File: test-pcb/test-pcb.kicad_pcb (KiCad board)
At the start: 4 copper layers, 16 parts, among them IC1 VNH5019ATR-E, J1 Conn_01x06, J2 Conn_01x06, J3 Conn_01x03, Q1 IPD050N10N5ATMA1

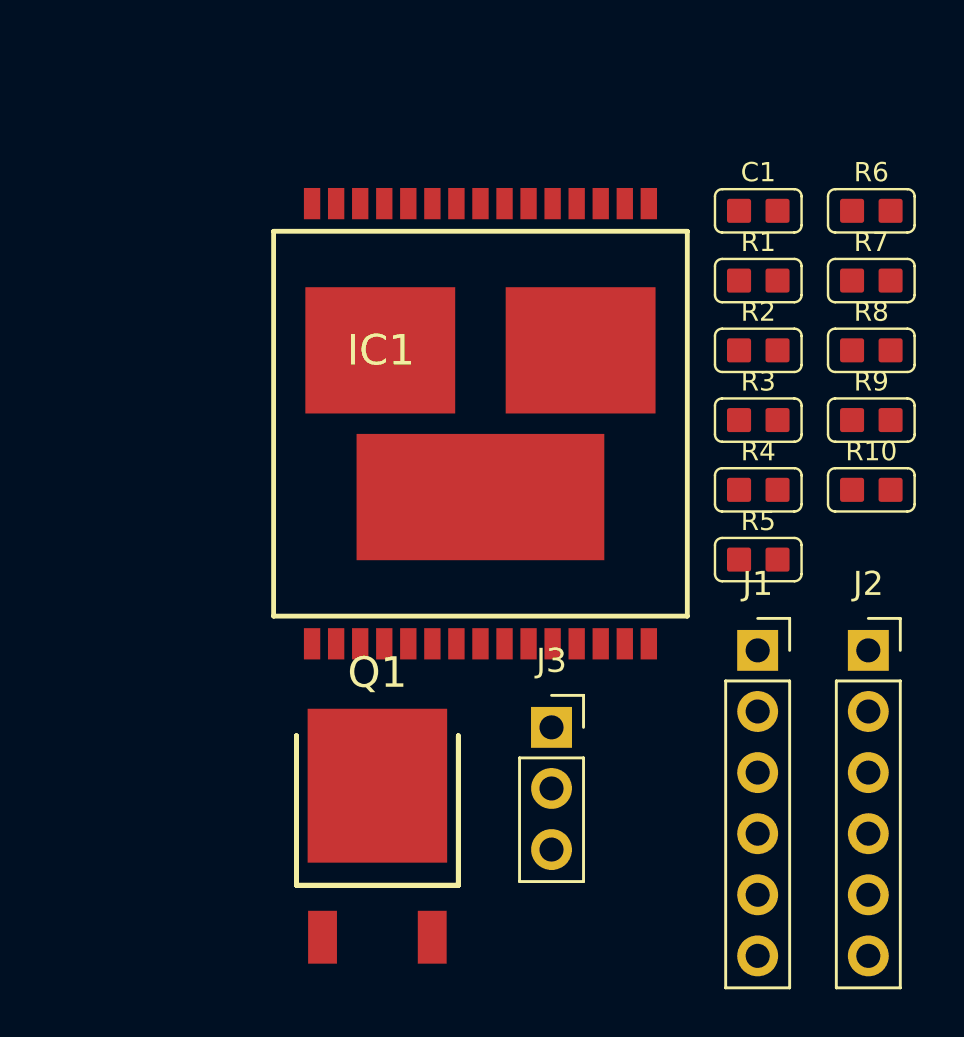
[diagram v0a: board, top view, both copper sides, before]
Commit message: test - thermal vias for driver
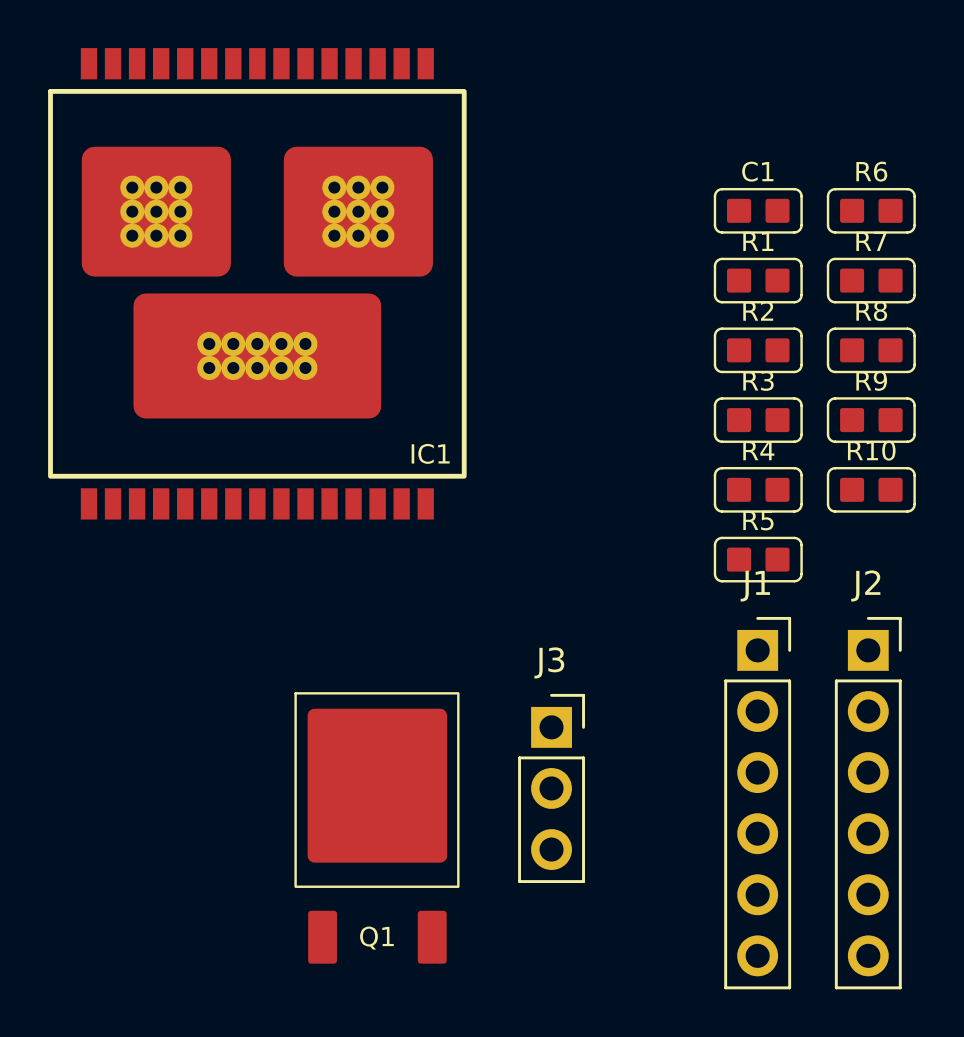
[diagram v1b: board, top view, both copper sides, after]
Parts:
- moved IC1 15.3 mm to (30.5, 35.6)

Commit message: test - fixed mdriver sch
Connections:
- IC1 pad GND: (no net) -> GND
- J2 pad 1: VCC -> /M1 OUTA
- J2 pad 6: GND -> /M1 OUTB
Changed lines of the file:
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@@
     (pad "24" smd rect (at -1 -9.15) (size 0.68 1.3) (layers "F.Cu" "F.Paste" "F.Mask"))
     (pad "29" smd rect (at -6 -9.15) (size 0.68 1.3) (layers "F.Cu" "F.Paste" "F.Mask"))
-    (pad "GND" smd rect (at -5 -9.15) (size 0.68 1.3) (layers "F.Cu" "F.Paste" "F.Mask"))
-    (pad "GND" smd rect (at -4 -9.15) (size 0.68 1.3) (layers "F.Cu" "F.Paste" "F.Mask"))
-    (pad "GND" smd rect (at -3 -9.15) (size 0.68 1.3) (layers "F.Cu" "F.Paste" "F.Mask"))
-    (pad "GND" smd rect (at 3 -9.15) (size 0.68 1.3) (layers "F.Cu" "F.Paste" "F.Mask"))
-    (pad "GND" smd rect (at 4 -9.15) (size 0.68 1.3) (layers "F.Cu" "F.Paste" "F.Mask"))
-    (pad "GND" smd rect (at 5 -9.15) (size 0.68 1.3) (layers "F.Cu" "F.Paste" "F.Mask"))
+    (pad "GND" smd rect (at -5 -9.15) (size 0.68 1.3) (layers "F.Cu" "F.Paste" "F.Mask")
+      (net 2 "GND") (pinfunction "GND") (pintype "passive"))
+    (pad "GND" smd rect (at -4 -9.15) (size 0.68 1.3) (layers "F.Cu" "F.Paste" "F.Mask")
+      (net 2 "GND") (pinfunction "GND") (pintype "passive"))
+    (pad "GND" smd rect (at -3 -9.15) (size 0.68 1.3) (layers "F.Cu" "F.Paste" "F.Mask")
+      (net 2 "GND") (pinfunction "GND") (pintype "passive"))
+    (pad "GND" smd rect (at 3 -9.15) (size 0.68 1.3) (layers "F.Cu" "F.Paste" "F.Mask")
+      (net 2 "GND") (pinfunction "GND") (pintype "passive"))
+    (pad "GND" smd rect (at 4 -9.15) (size 0.68 1.3) (layers "F.Cu" "F.Paste" "F.Mask")
+      (net 2 "GND") (pinfunction "GND") (pintype "passive"))
+    (pad "GND" smd rect (at 5 -9.15) (size 0.68 1.3) (layers "F.Cu" "F.Paste" "F.Mask")
+      (net 2 "GND") (pinfunction "GND") (pintype "passive"))
     (pad "OUTA" smd rect (at -7 -9.15) (size 0.68 1.3) (layers "F.Cu" "F.Paste" "F.Mask")
       (net 12 "/M1 OUTA") (pinfunction "OUTA") (pintype "passive"))
@@
       (stroke (width 0.1) (type solid)) (layer "F.Fab"))
     (pad "1" thru_hole rect (at 0 0) (size 1.7 1.7) (drill 1) (layers "*.Cu" "*.Mask")
-      (net 11 "VCC") (pinfunction "Pin_1") (pintype "passive"))
+      (net 12 "/M1 OUTA") (pinfunction "Pin_1") (pintype "passive"))
     (pad "2" thru_hole oval (at 0 2.54) (size 1.7 1.7) (drill 1) (layers "*.Cu" "*.Mask")
       (net 2 "GND") (pinfunction "Pin_2") (pintype "passive"))
@@
       (net 20 "+3V3") (pinfunction "Pin_5") (pintype "passive"))
     (pad "6" thru_hole oval (at 0 12.7) (size 1.7 1.7) (drill 1) (layers "*.Cu" "*.Mask")
-      (net 2 "GND") (pinfunction "Pin_6") (pintype "passive"))
+      (net 13 "/M1 OUTB") (pinfunction "Pin_6") (pintype "passive"))
     (model "${KICAD6_3DMODEL_DIR}/Connector_PinSocket_2.54mm.3dshapes/PinSocket_1x06_P2.54mm_Vertical.wrl"
       (offset (xyz 0 0 0))
